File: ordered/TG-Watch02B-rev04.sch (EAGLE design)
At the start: 66 parts, among them IC3 W25Q128JVSIQ TR, J1 USB-C-CON-TG_MOD-2295018-2.0, J2 DISP_1.54_LCMTF15423A-C_LCD+C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, J3 CON-BAT-TG-MEZ_FEMALE, Q3 DMG2305, U2 MICROBUILDER_LSM6DSOX, U3 VREG-TPS63036, U4 FAN5331SX, U5 MCP73831/OT, U6 LC709203F, U8 UNDERVOLT-TPS3702CX3

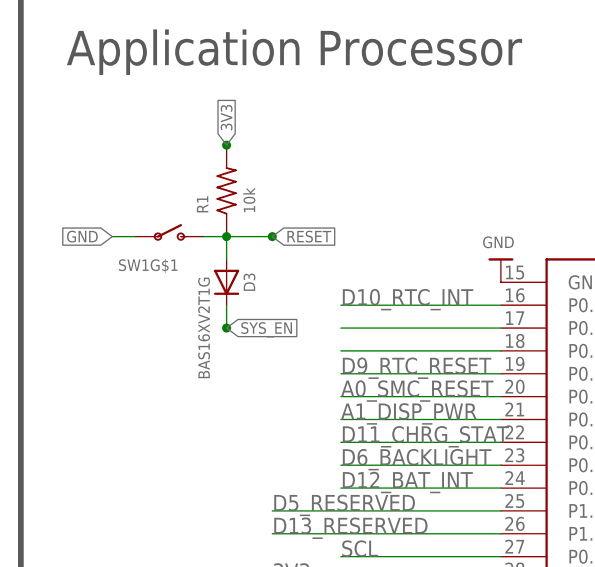
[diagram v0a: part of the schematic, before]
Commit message: pre-order
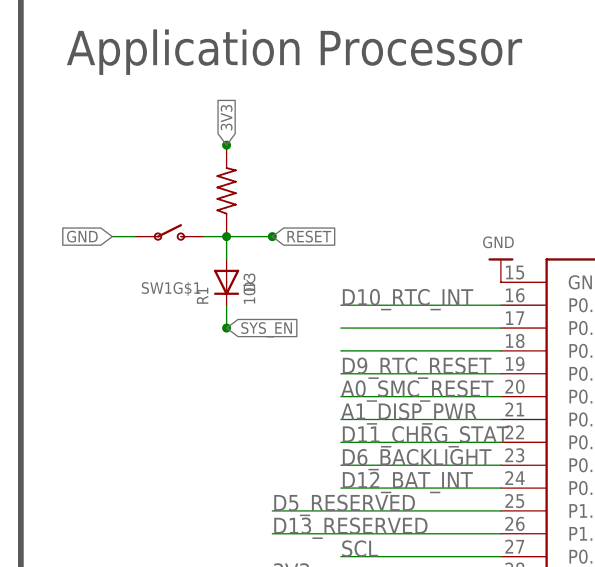
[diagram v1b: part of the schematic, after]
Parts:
- D3: value BAS16XV2T1G -> (none)
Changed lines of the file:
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@@
 <part name="R13" library="0TG-Lib v01.5" deviceset="R_TG" device="_0402" value="10k"/>
 <part name="U$3" library="0TG-Lib v01.5" deviceset="CON_SWD_POGO" device=""/>
-<part name="D3" library="0TG-Lib v01.5" deviceset="DIODE" device="SOD-523" value="BAS16XV2T1G"/>
+<part name="D3" library="0TG-Lib v01.5" deviceset="DIODE" device="SOD-523"/>
 <part name="R1" library="0TG-Lib v01.5" deviceset="R_TG" device="_0402" value="10k"/>
 <part name="C2" library="0TG-Lib v01.5" deviceset="C-US_" device="_0402_NOMASK" value="10uf"/>
@@
 <instance part="D3" gate="G$1" x="58.42" y="205.74" smashed="yes" rot="R270">
 <attribute name="NAME" x="60.96" y="205.74" size="1.27" layer="95" rot="R270" align="center"/>
-<attribute name="VALUE" x="55.92" y="200.66" size="1.27" layer="96" rot="R270" align="center"/>
+<attribute name="VALUE" x="55.92" y="205.74" size="1.27" layer="96" rot="R270" align="center"/>
 </instance>
 <instance part="R1" gate="A" x="58.42" y="215.9" smashed="yes" rot="R90">
-<attribute name="NAME" x="56.388" y="213.36" size="1.27" layer="95" font="vector" rot="R90"/>
-<attribute name="VALUE" x="61.595" y="213.36" size="1.27" layer="96" font="vector" rot="R90"/>
+<attribute name="NAME" x="56.388" y="203.2" size="1.27" layer="95" font="vector" rot="R90"/>
+<attribute name="VALUE" x="61.595" y="203.2" size="1.27" layer="96" font="vector" rot="R90"/>
 </instance>
 <instance part="C2" gate="G$1" x="147.32" y="25.4" smashed="yes" rot="R180">
@@
 </instance>
 <instance part="SW1" gate="G$1" x="53.34" y="210.82" smashed="yes">
-<attribute name="NAME" x="46.355" y="207.01" size="1.27" layer="95"/>
+<attribute name="NAME" x="48.895" y="204.47" size="1.27" layer="95"/>
 <attribute name="VALUE" x="48.26" y="214.63" size="1.27" layer="96"/>
 </instance>
